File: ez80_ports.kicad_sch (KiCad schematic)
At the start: 18 parts

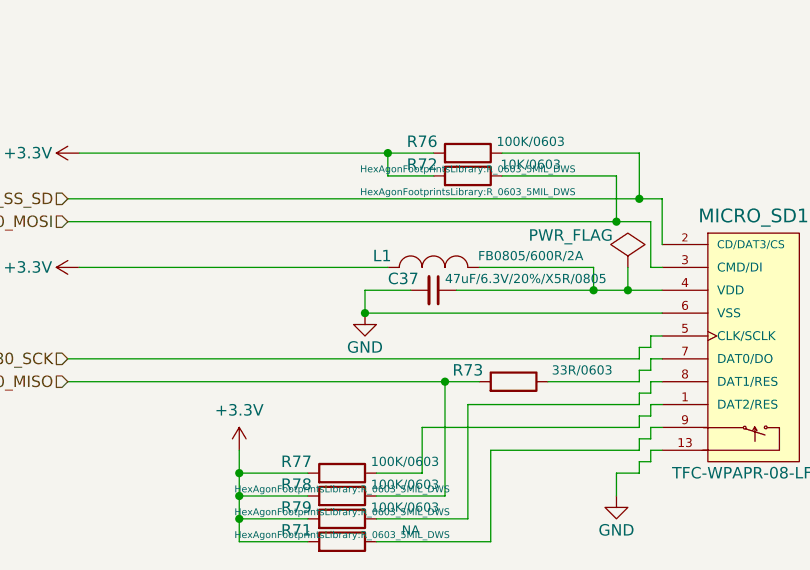
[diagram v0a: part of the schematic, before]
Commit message: v1.0 version PCB
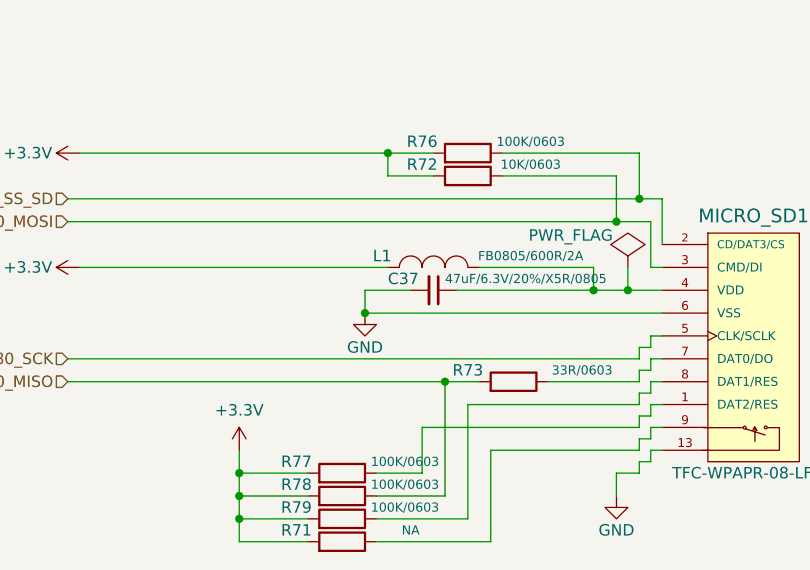
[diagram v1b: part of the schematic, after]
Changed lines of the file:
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@@
 					(size 0.762 0.762)
 				)
+				(hide yes)
 			)
 		)
@@
 					(size 0.762 0.762)
 				)
+				(hide yes)
 			)
 		)
@@
 					(size 0.762 0.762)
 				)
+				(hide yes)
 			)
 		)
@@
 					(size 0.762 0.762)
 				)
+				(hide yes)
 			)
 		)
@@
 					(size 0.762 0.762)
 				)
-			)
-		)
+				(hide yes)
+			)
+		)

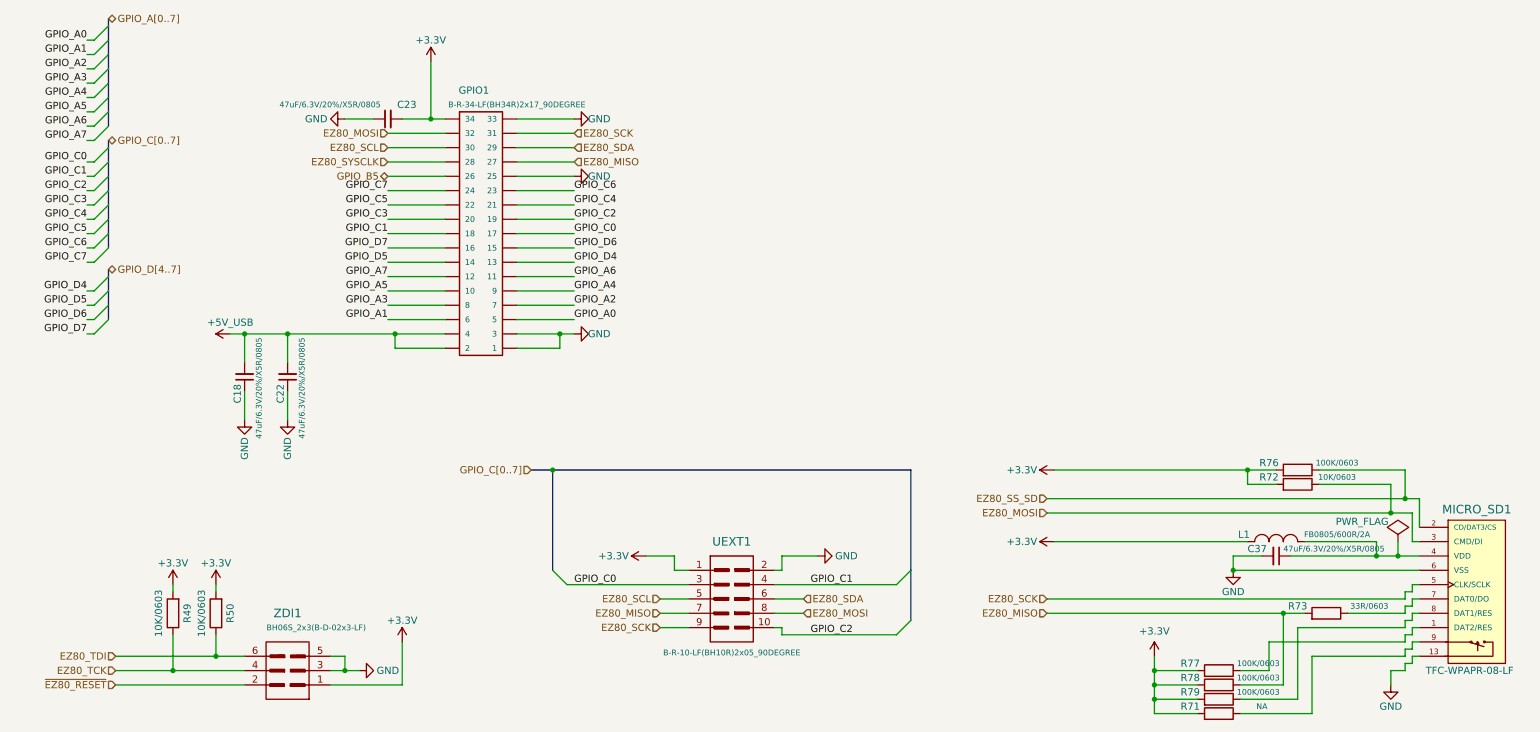
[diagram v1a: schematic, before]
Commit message: 1st production and BOM
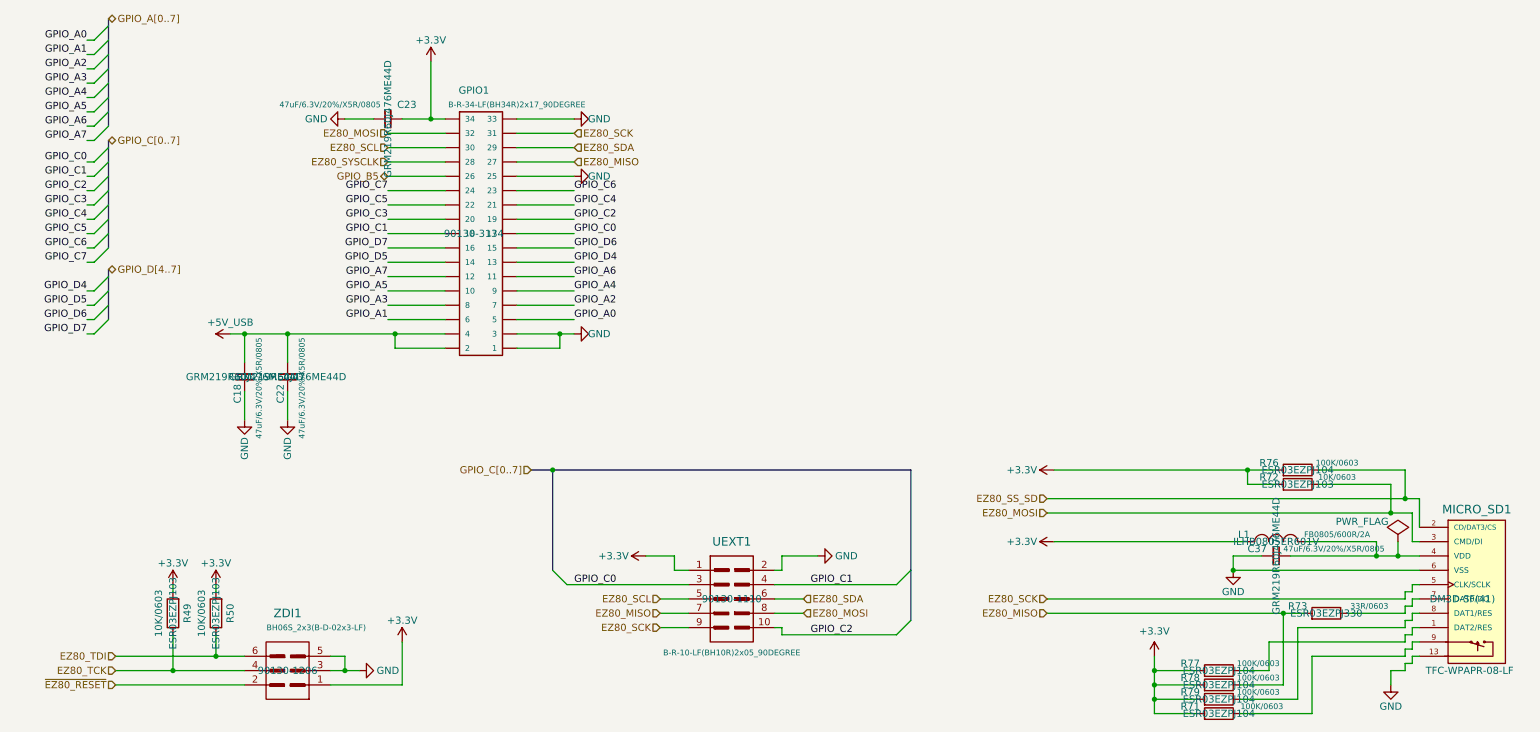
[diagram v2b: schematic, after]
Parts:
- C18, C22, C23, C37: MfgNumber (none) -> GRM219R60J476ME44D
- GPIO1: MfgNumber (none) -> 90130-3134
- L1: MfgNumber (none) -> ILHB0805ER601V
- MICRO_SD1: MfgNumber (none) -> DM3D-SF(41)
- R49, R50, R72: MfgNumber (none) -> ESR03EZPJ103
- R71: value NA -> 100K/0603; MfgNumber (none) -> ESR03EZPJ104
- R73: MfgNumber (none) -> ESR03EZPJ330
- R76, R77, R78, R79: MfgNumber (none) -> ESR03EZPJ104
- UEXT1: MfgNumber (none) -> 90130-1110
- ZDI1: MfgNumber (none) -> 90130-1206
